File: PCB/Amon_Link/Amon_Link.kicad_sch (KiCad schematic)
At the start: 98 parts, among them IC1 SPX5205M5-L/TR, J1 USB_C_Receptacle_USB2.0, J2 SMA Edge, J3 Programing port, J4 SMA Edge, SW1 SW_SPST, U1 CH32V003F4P6, U2 CH340G, U3 NRF24L01, U4 RFX2401C, U5 NRF24L01, U6 RFX2401C, Y1 12MHz, Y2 12MHz, Y3 16MHz, Y4 16MHz

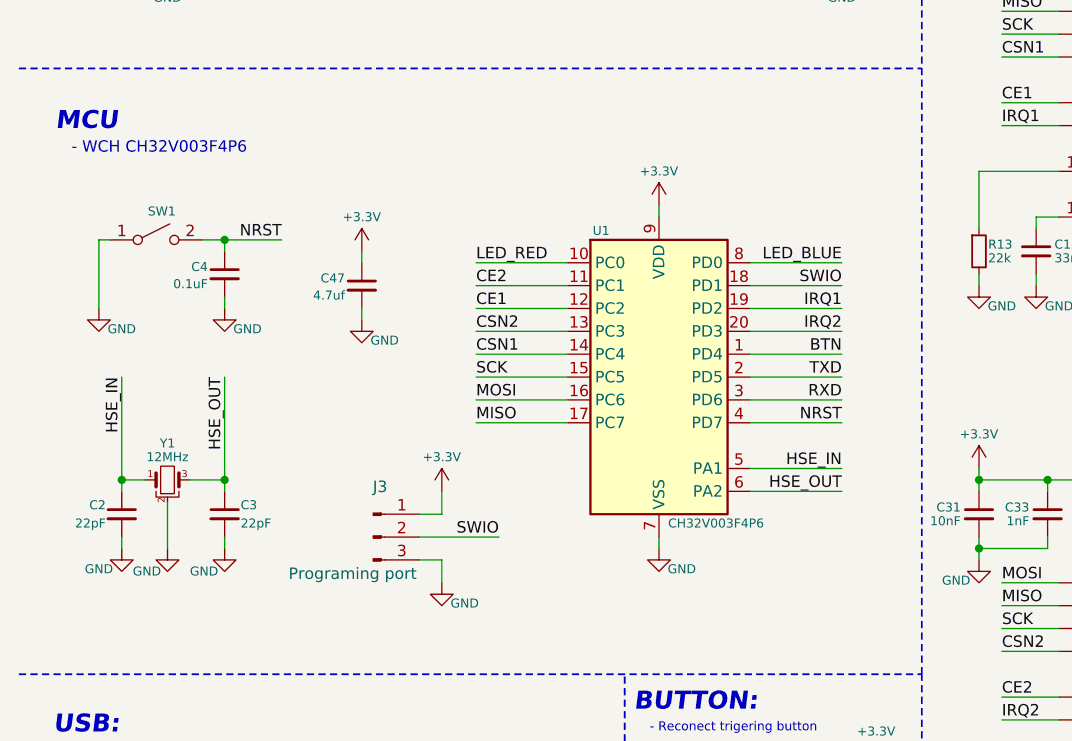
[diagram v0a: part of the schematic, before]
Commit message: pcb update and case
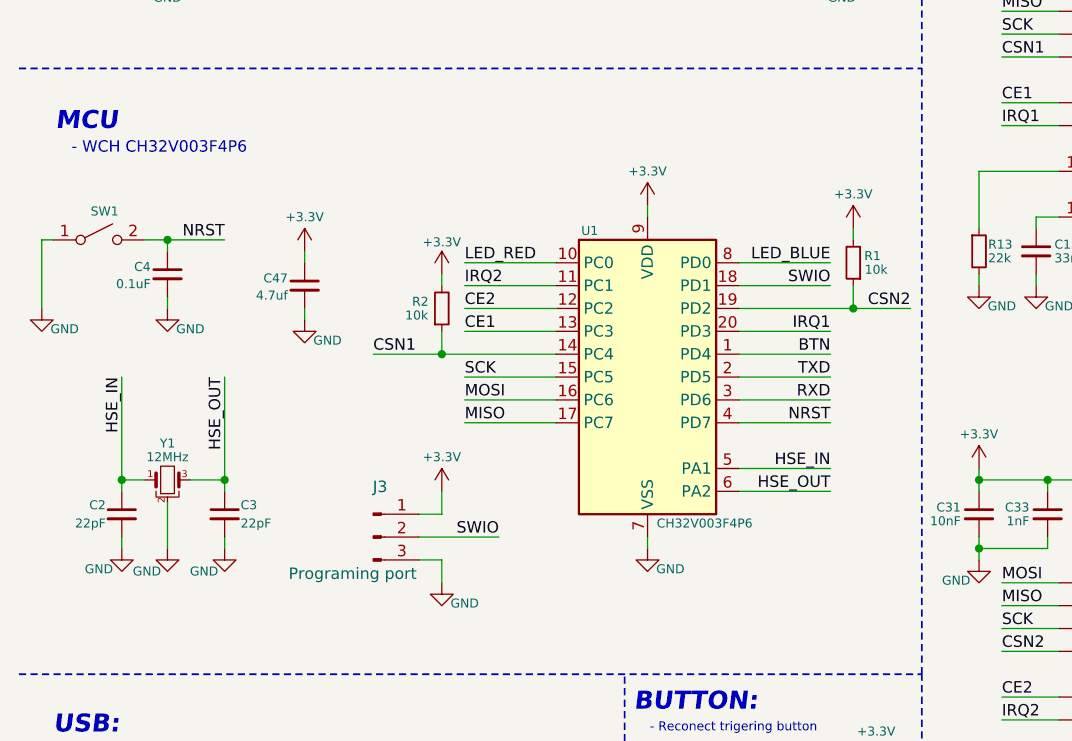
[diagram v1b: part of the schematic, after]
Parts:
- added R1, R2: 10k, Resistor_SMD:R_0603_1608Metric, symbol Device:R_Small
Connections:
- net +3.3V: now also R1.2, R2.2
- net CE1: now also U1.13 (PC3); no longer U1.12 (PC2)
- net CE2: now also U1.12 (PC2); no longer U1.11 (PC1)
- net CSN1: now also R2.1
- net CSN2: now also U1.19 (PD2), R1.1; no longer U1.13 (PC3)
- net IRQ1: now also U1.20 (PD3); no longer U1.19 (PD2)
- net IRQ2: now also U1.11 (PC1); no longer U1.20 (PD3)
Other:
- moved on the sheet: C4, C47, SW1, U1
